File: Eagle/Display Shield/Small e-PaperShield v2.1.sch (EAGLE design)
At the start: 116 parts, among them J2 3300060P1-ST-TF-003A, J3 2.54-8p-male-SMD, J4 2.54-8p-male-SMD, J5 2.54-6p-male-SMD, J6 2.54-6p-male-SMD, J7 2.54-2x3p-female-SMD, Q10 MOSFET-P-044021001, Q11 2N7002, Q2 2N7002, Q3 MOSFET-P-044021001, Q5 MOSFET-P-044021001, Q7 MOSFET-P-044021001, Q8 2N7002, Q9 2N7002, U2 XC6206-3.3-1300260P1, U3 74VHC125PW, U4 74VHC125PW, U5 GT20L16P1Y, U9 S-8120CNB-DRB-TF-G//200021001, X1 FH12-40S-0.5SH

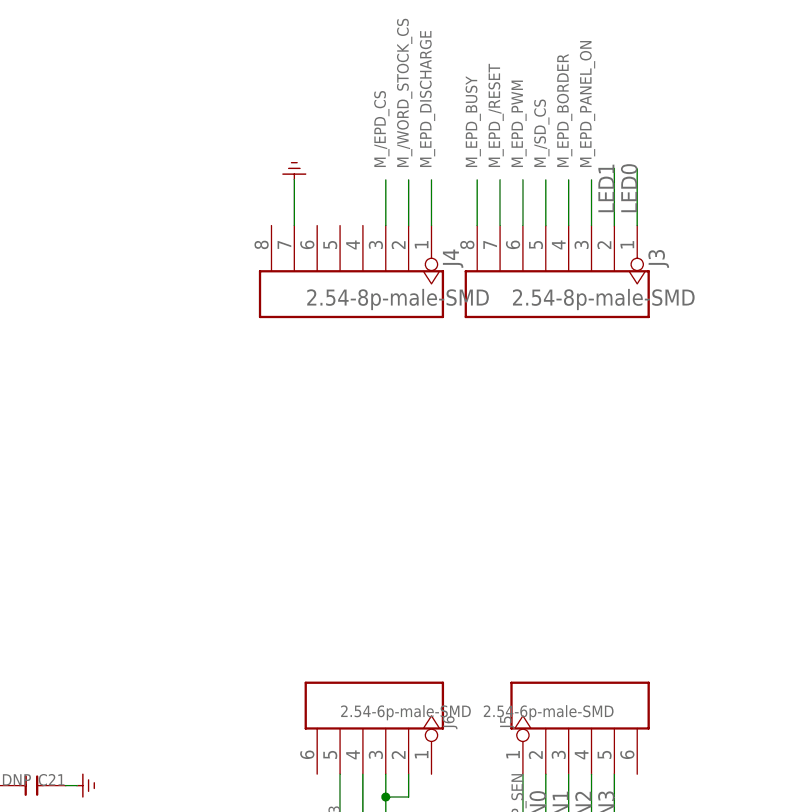
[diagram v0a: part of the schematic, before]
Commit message: finished display shield
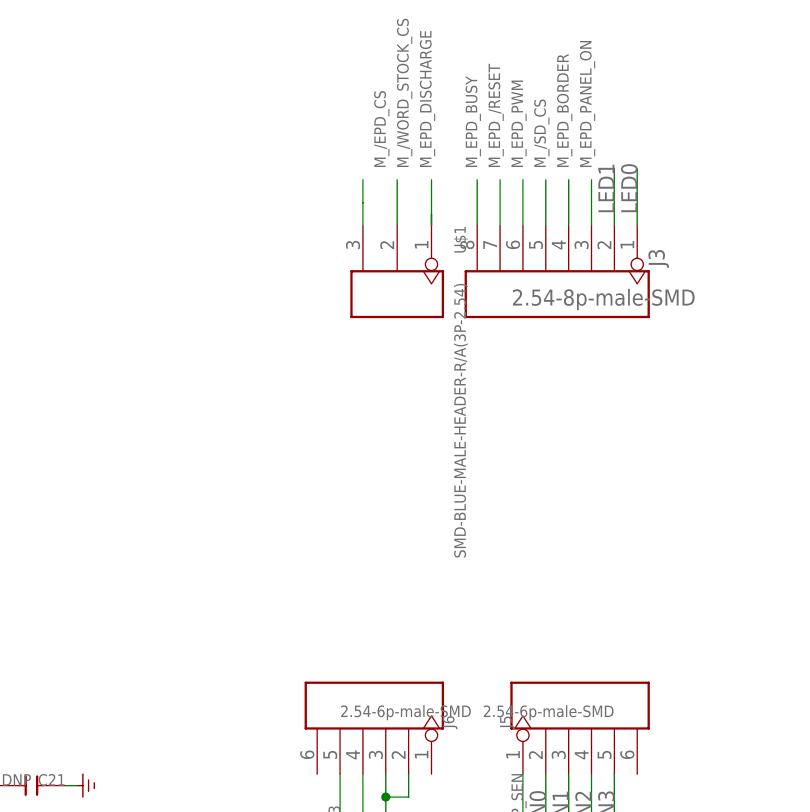
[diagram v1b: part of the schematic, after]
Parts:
- removed J4: 2.54-8p-male-SMD, Connector:HEADER-8P-2.54-SMD
- added U$1: SMD-BLUE-MALE-HEADER-R/A(3P-2.54), Seeed-OPL-Connector:SMD-BLUE-MALE-HEADER-R/A(3P-2.54)
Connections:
- net GND: no longer J4.7
- net M_/EPD_CS: now also U$1.P$3; no longer J4.3
- net M_/WORD_STOCK_CS: now also U$1.P$2; no longer J4.2
- net M_EPD_DISCHARGE: now also U$1.P$1; no longer J4.1
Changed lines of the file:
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@@
 <setting verticaltext="up"/>
 </settings>
-<grid distance="0.1" unitdist="inch" unit="inch" style="lines" multiple="1" display="no" altdistance="0.01" altunitdist="inch" altunit="inch"/>
+<grid distance="0.05" unitdist="inch" unit="inch" style="lines" multiple="1" display="no" altdistance="0.01" altunitdist="inch" altunit="inch"/>
 <layers>
 <layer number="1" name="Top" color="4" fill="1" visible="no" active="no"/>
@@
 <layer number="112" name="tSilk" color="7" fill="1" visible="no" active="no"/>
 <layer number="113" name="IDFDebug" color="4" fill="1" visible="no" active="yes"/>
+<layer number="114" name="FRNTMAAT1" color="7" fill="1" visible="yes" active="yes"/>
+<layer number="115" name="FRNTMAAT2" color="7" fill="1" visible="yes" active="yes"/>
 <layer number="116" name="Patch_BOT" color="7" fill="1" visible="no" active="no"/>
+<layer number="117" name="BACKMAAT1" color="7" fill="1" visible="yes" active="yes"/>
 <layer number="118" name="Rect_Pads" color="7" fill="1" visible="no" active="no"/>
+<layer number="119" name="KAP_TEKEN" color="7" fill="1" visible="yes" active="yes"/>
+<layer number="120" name="KAP_MAAT1" color="7" fill="1" visible="yes" active="yes"/>
 <layer number="121" name="_tsilk" color="7" fill="1" visible="no" active="no"/>
 <layer number="122" name="_bsilk" color="7" fill="1" visible="no" active="no"/>
@@
 <layer number="131" name="tAdjust" color="7" fill="1" visible="no" active="no"/>
 <layer number="132" name="bAdjust" color="7" fill="1" visible="no" active="no"/>
+<layer number="133" name="bottom_silk" color="7" fill="1" visible="yes" active="yes"/>
 <layer number="144" name="DrillLegend" color="7" fill="1" visible="no" active="no"/>
 <layer number="145" name="DrillLegend_01-16" color="2" fill="9" visible="yes" active="yes"/>
@@
 <layer number="223" name="223bmp" color="24" fill="1" visible="no" active="no"/>
 <layer number="224" name="224bmp" color="25" fill="1" visible="no" active="no"/>
+<layer number="225" name="225bmp" color="7" fill="1" visible="no" active="no"/>
+<layer number="226" name="226bmp" color="7" fill="1" visible="no" active="no"/>
+<layer number="227" name="227bmp" color="7" fill="1" visible="no" active="no"/>
+<layer number="228" name="228bmp" color="7" fill="1" visible="no" active="no"/>
+<layer number="229" name="229bmp" color="7" fill="1" visible="yes" active="yes"/>
+<layer number="230" name="230bmp" color="7" fill="1" visible="no" active="no"/>
 <layer number="231" name="Eagle3D_PG1" color="14" fill="1" visible="yes" active="yes"/>
 <layer number="232" name="Eagle3D_PG2" color="14" fill="2" visible="yes" active="yes"/>
@@
 <layer number="251" name="SMDround" color="12" fill="11" visible="no" active="no"/>
 <layer number="254" name="OrgLBR" color="13" fill="1" visible="no" active="no"/>
+<layer number="255" name="Accent" color="7" fill="1" visible="yes" active="yes"/>
 </layers>
 <schematic xreflabel="%F%N/%S.%C%R" xrefpart="/%S.%C%R">
@@
 <part name="U$6" library="Power or GND " deviceset="GND_POWER" device=""/>
 <part name="U$7" library="Power or GND " deviceset="GND_POWER" device=""/>
-<part name="U$8" library="Power or GND " deviceset="GND_POWER" device=""/>
 <part name="U3" library="IC" deviceset="74V*125" device="PW" technology="HC"/>
 <part name="J2" library="OPL-NEW" deviceset="3300060P1-ST-TF-003A" device=""/>
@@
 <part name="U$46" library="Power or GND " deviceset="GND_POWER" device=""/>
 <part name="J3" library="Connector" deviceset="HEADER-8P" device="-2.54-SMD" value="2.54-8p-male-SMD"/>
-<part name="J4" library="Connector" deviceset="HEADER-8P" device="-2.54-SMD" value="2.54-8p-male-SMD"/>
 <part name="J5" library="Connector" deviceset="HEADER-6P" device="-SMD" value="2.54-6p-male-SMD"/>
 <part name="J6" library="Connector" deviceset="HEADER-6P" device="-SMD" value="2.54-6p-male-SMD"/>
@@
 <part name="R17" library="Discrete" deviceset="R*" device="-0603" value="10k"/>
 <part name="JP1" library="SparkFun-Connectors" deviceset="M05" device="PTH_LONGPADS"/>
+<part name="U$1" library="Seeed-OPL-Connector" deviceset="SMD-BLUE-MALE-HEADER-R/A(3P-2.54)" device=""/>
 </parts>
 <sheets>
@@
 <instance part="U$6" gate="G$1" x="-215.9" y="96.52"/>
 <instance part="U$7" gate="G$1" x="445.77" y="71.12"/>
-<instance part="U$8" gate="G$1" x="435.61" y="142.24" rot="R180"/>
 <instance part="U3" gate="A" x="38.1" y="147.32"/>
 <instance part="U3" gate="PWR" x="38.1" y="158.75" smashed="yes" rot="R270">
@@
 <instance part="U$46" gate="G$1" x="-55.88" y="154.94" rot="R270"/>
 <instance part="J3" gate="J" x="464.82" y="129.54" rot="R270"/>
-<instance part="J4" gate="J" x="441.96" y="129.54" rot="R270"/>
 <instance part="J5" gate="J" x="467.36" y="83.82" rot="R90"/>
 <instance part="J6" gate="J" x="444.5" y="83.82" rot="MR90"/>
@@
 <instance part="R17" gate="R" x="295.91" y="81.28" rot="MR0"/>
 <instance part="JP1" gate="G$1" x="345.44" y="160.02" rot="R180"/>
+<instance part="U$1" gate="G$1" x="447.04" y="129.54" rot="R270"/>
 </instances>
 <busses>
@@
 <pinref part="J6" gate="J" pin="2"/>
 <pinref part="J6" gate="J" pin="3"/>
-</segment>
-<segment>
-<wire x1="435.61" y1="137.16" x2="435.61" y2="142.24" width="0.1524" layer="91"/>
-<pinref part="U$8" gate="G$1" pin="GND"/>
-<pinref part="J4" gate="J" pin="7"/>
 </segment>
 <segment>
@@
 <net name="M_EPD_DISCHARGE" class="0">
 <segment>
-<wire x1="450.85" y1="137.16" x2="450.85" y2="142.24" width="0.1524" layer="91"/>
 <label x="450.85" y="143.51" size="1.27" layer="95" ratio="10" rot="R90"/>
-<pinref part="J4" gate="J" pin="1"/>
+<wire x1="450.85" y1="142.24" x2="450.85" y2="137.16" width="0.1524" layer="91"/>
+<pinref part="U$1" gate="G$1" pin="P$1"/>
 </segment>
 <segment>
@@
 <net name="M_/EPD_CS" class="0">
 <segment>
-<wire x1="445.77" y1="137.16" x2="445.77" y2="142.24" width="0.1524" layer="91"/>
 <label x="445.77" y="143.51" size="1.27" layer="95" ratio="10" rot="R90"/>
-<pinref part="J4" gate="J" pin="3"/>
+<wire x1="443.23" y1="139.7" x2="443.23" y2="142.24" width="0.1524" layer="91"/>
+<wire x1="443.23" y1="139.7" x2="443.23" y2="137.16" width="0.1524" layer="91"/>
+<pinref part="U$1" gate="G$1" pin="P$3"/>
 </segment>
 <segment>
@@
 <net name="M_/WORD_STOCK_CS" class="0">
 <segment>
-<wire x1="448.31" y1="137.16" x2="448.31" y2="142.24" width="0.1524" layer="91"/>
 <label x="448.31" y="143.51" size="1.27" layer="95" ratio="10" rot="R90"/>
-<pinref part="J4" gate="J" pin="2"/>
+<pinref part="U$1" gate="G$1" pin="P$2"/>
+<wire x1="447.04" y1="142.24" x2="447.04" y2="137.16" width="0.1524" layer="91"/>
 </segment>
 <segment>
@@
 </segment>
 </net>
+<net name="N$15" class="0">
+<segment>
+<wire x1="450.85" y1="137.16" x2="450.85" y2="138.43" width="0.1524" layer="91"/>
+</segment>
+</net>
